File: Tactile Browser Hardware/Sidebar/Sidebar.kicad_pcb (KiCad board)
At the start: 2 copper layers, 230.8 x 22.8 mm, 40 parts, among them J1 Conn_01x02_Pin, J2 Conn_01x02_Pin, J3 Barrel_Jack_Switch, J4 Conn_01x02_Pin, Q1 PMOS, SW10 SW_Push, SW11 SW_Push, SW12 SW_Push, SW6 SW_Push, SW7 SW_Push, SW8 SW_Push, SW9 SW_Push

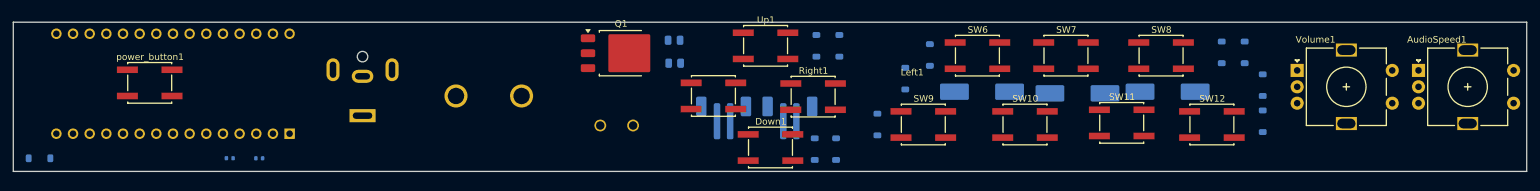
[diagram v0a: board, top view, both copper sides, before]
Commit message: sidebar pcb progress
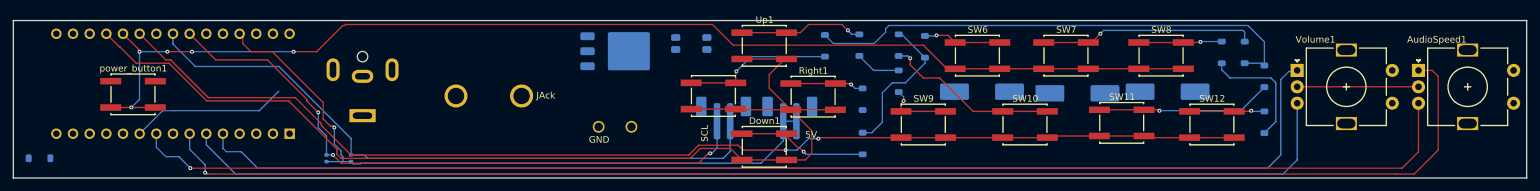
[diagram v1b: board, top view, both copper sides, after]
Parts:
- Q1: moved to B.Cu
- moved 4.7k_ohm2 14.8 mm to (76.5, 72.8), turned to -90 degrees
- moved 4.7k_ohm1 14.0 mm to (80.2, 72.8), turned to 90 degrees
- moved D4 8.61 mm to (158.2, 63.8), turned to 90 degrees
- moved D9 7.36 mm to (163.8, 61.0), turned to -90 degrees
- moved D2 7.35 mm to (158.2, 70.5)
- moved 100kR1 5.76 mm to (134.5, 55.2), turned to -90 degrees
- moved D10 5.20 mm to (163.8, 55.5)
- moved power_button1 3.09 mm to (47.0, 63.0)
- moved D1 3.05 mm to (157.8, 55.5)
- moved D6 1.46 mm to (167.8, 55.8)
- moved D11 1.37 mm to (219.5, 60.2)
- moved D3 1.30 mm to (152.5, 55.6)
- moved Down1 0.96 mm to (143.2, 71.0)
- moved 1kR1 0.56 mm to (129.8, 55.2), turned to -90 degrees
- moved J2 0.32 mm to (118.0, 68.0)
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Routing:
- net AS1: track 0.00 -> 211.1 mm, vias 0 -> 1
- net AS2: track 0.00 -> 204.3 mm, vias 0 -> 1
- net Col2: track 0.00 -> 183.3 mm, vias 0 -> 5
- net RE1: track 0.00 -> 180.2 mm
- net RE2: track 0.00 -> 179.4 mm
- net Col3: track 0.00 -> 176.6 mm, vias 0 -> 2
- net Col1: track 0.00 -> 165.6 mm
- net 5V: track 0.00 -> 104.4 mm, vias 0 -> 1
- net SDA: track 0.00 -> 100.2 mm
- net SCL: track 0.00 -> 96.9 mm, vias 0 -> 3
- net Row3: track 0.00 -> 76.8 mm
- net Net-(D7-A): track 0.00 -> 33.0 mm, vias 0 -> 1
- net Row1: track 0.00 -> 30.8 mm
- net Net-(D10-A): track 0.00 -> 26.7 mm, vias 0 -> 1
- net Net-(D11-A): track 0.00 -> 26.7 mm, vias 0 -> 1
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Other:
- board size 230.8 x 22.8 mm -> 230.8 x 24 mm
- board text added: "5V"
- board text added: "GND"
- board text added: "JAck"
- board text added: "SCL"
